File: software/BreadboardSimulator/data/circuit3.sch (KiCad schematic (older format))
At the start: 16 parts, among them Q1 Transistor, SW1 SwitchPush, U1-8 8pinChip

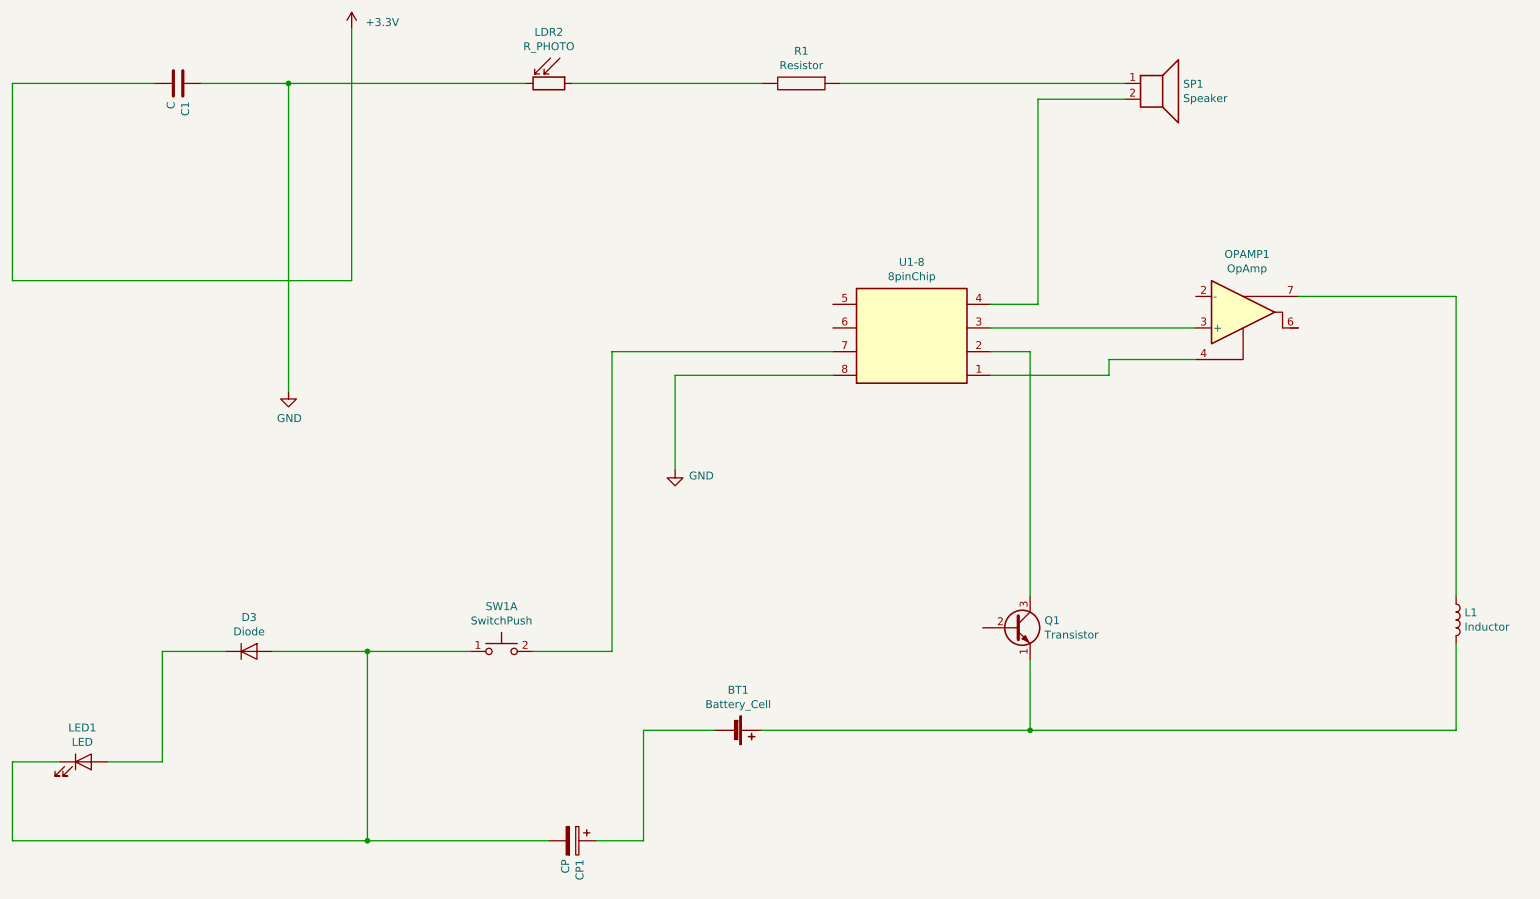
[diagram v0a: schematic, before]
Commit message: In progress: travel net lists
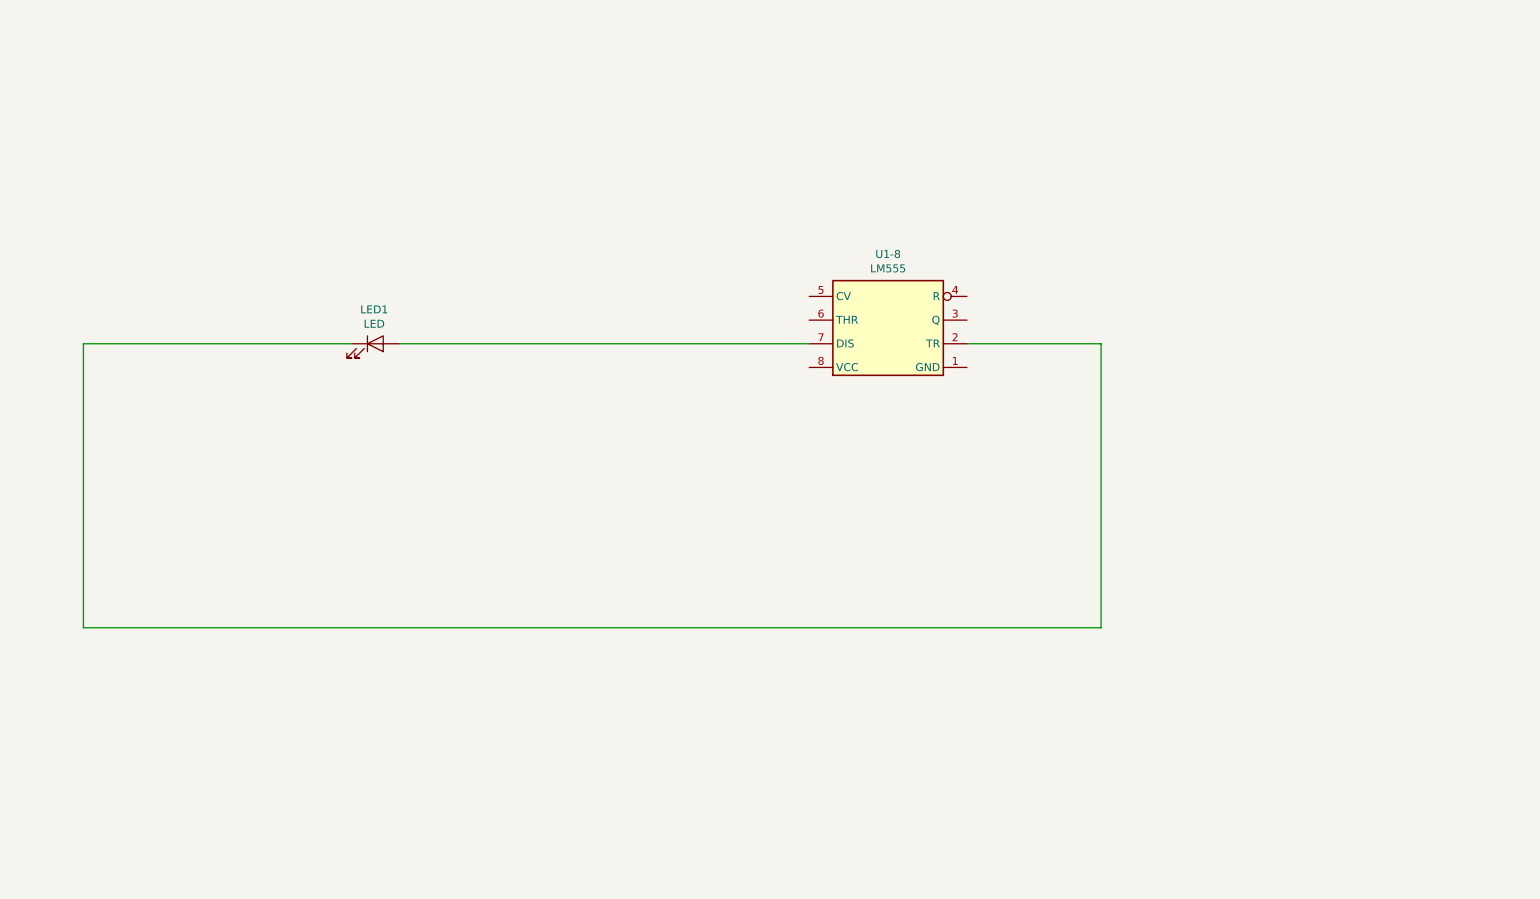
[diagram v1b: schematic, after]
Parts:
- removed BT1: Battery_Cell, symbol SchemaBoard_Library:Battery_Cell
- removed C1: C, symbol SchemaBoard_Library:C
- removed CP1: CP, symbol SchemaBoard_Library:CP
- removed D3: Diode, symbol SchemaBoard_Library:Diode
- removed GND1, GND2: GND, symbol SchemaBoard_Library:GND
- removed L1: Inductor, symbol SchemaBoard_Library:Inductor
- removed LDR2: R_PHOTO, symbol SchemaBoard_Library:R_PHOTO
- removed OPAMP1: OpAmp, symbol SchemaBoard_Library:OpAmp
- removed PWR1: +3.3V, symbol SchemaBoard_Library:+3.3V
- removed Q1: Transistor, symbol SchemaBoard_Library:Transistor
- removed R1: Resistor, symbol SchemaBoard_Library:Resistor
- removed SP1: Speaker, symbol SchemaBoard_Library:Speaker
- removed SW1: SwitchPush, symbol SchemaBoard_Library:SwitchPush
- removed U1-8: 8pinChip, symbol SchemaBoard_Library:8pinChip
- added U1-8: LM555, symbol SchemaBoard_Library:LM555
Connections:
- net at LED1.2 (A): now also U1-8.7 (DIS)
- net at LED1.1 (K): now also U1-8.2 (TR)
